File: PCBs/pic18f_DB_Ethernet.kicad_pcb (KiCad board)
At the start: 2 copper layers, 100 x 98 mm, 40 parts, among them J1 OC1, J2 PicKIT 3, J3 IC1, J4 FC1, J5 MC1, J6 DB9_Female, J7 DB9_Male, J8 RJ45, SW1 SW_DPDT_x2, SW2 PWR_SW, U1 pic18f45k20

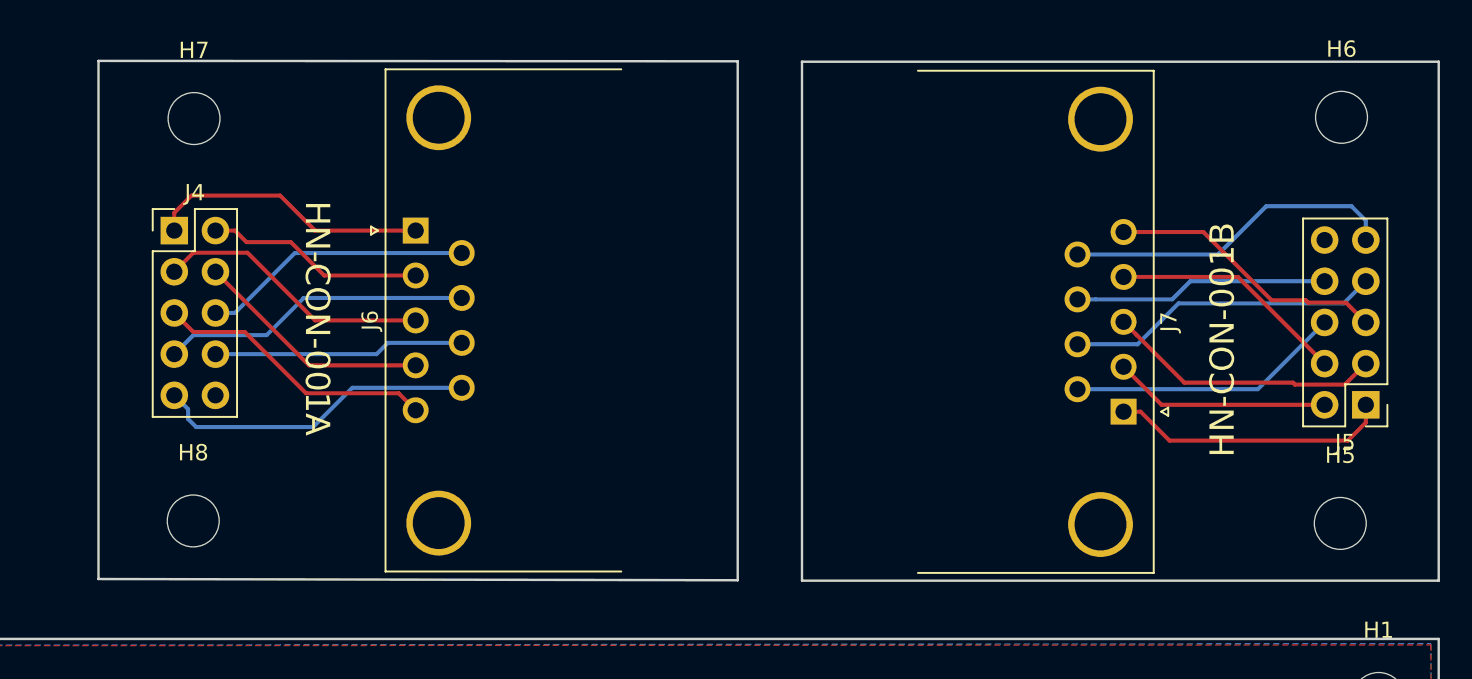
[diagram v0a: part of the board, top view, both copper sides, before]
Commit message: Restructed project
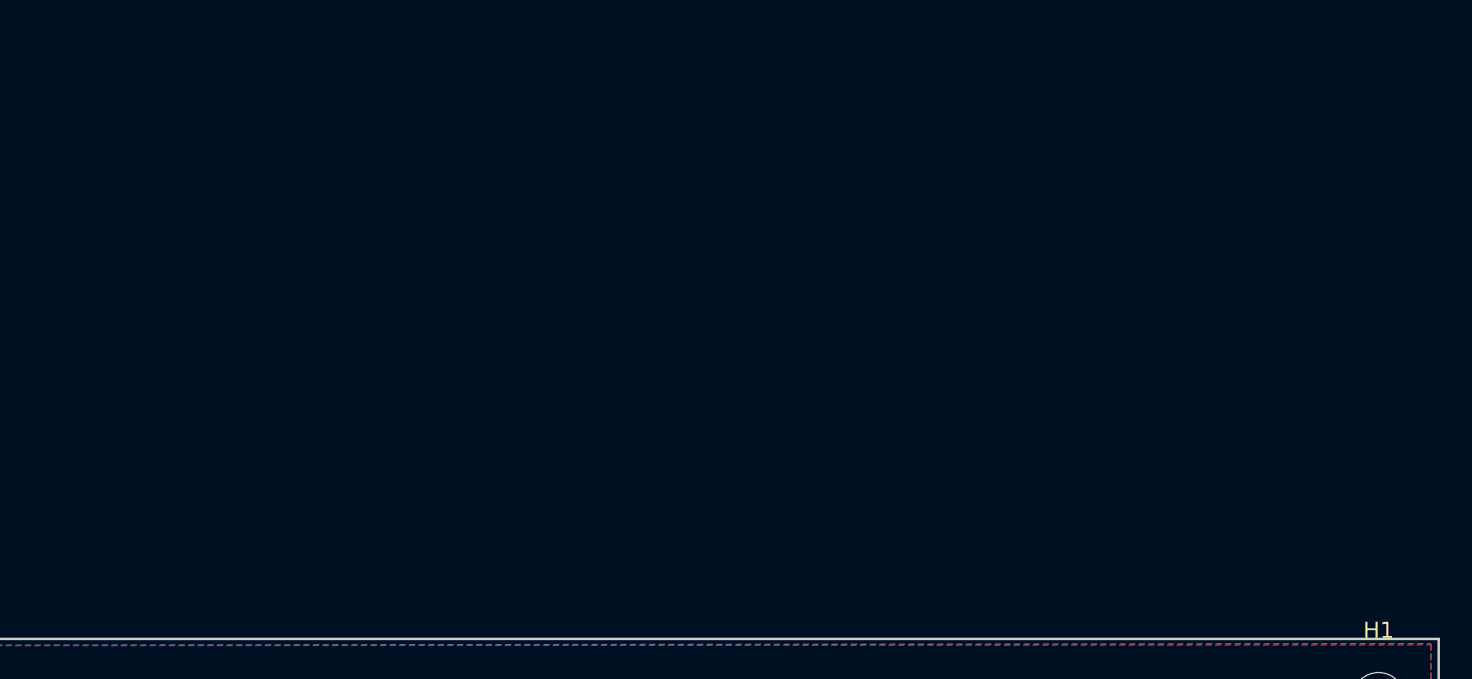
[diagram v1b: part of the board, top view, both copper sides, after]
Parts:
- removed H5, H6, H7, H8: MountingHole, MountingHole:MountingHole_3.2mm_M3
- removed J4: FC1, Connector_PinHeader_2.54mm:PinHeader_2x05_P2.54mm_Vertical
- removed J5: MC1, Connector_PinHeader_2.54mm:PinHeader_2x05_P2.54mm_Vertical
- removed J6: DB9_Female, Connector_Dsub:DSUB-9_Female_Horizontal_P2.77x2.84mm_EdgePinOffset9.90mm_Housed_MountingHolesOffset11.32mm
- removed J7: DB9_Male, Connector_Dsub:DSUB-9_Female_Horizontal_P2.77x2.84mm_EdgePinOffset9.90mm_Housed_MountingHolesOffset11.32mm
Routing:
- net M9: track 20.6 -> 0.00 mm
- net F9: track 19.9 -> 0.00 mm
- net M7: track 19.4 -> 0.00 mm
- net F7: track 19.2 -> 0.00 mm
- net F5: track 17.4 -> 0.00 mm
- net F1: track 17.3 -> 0.00 mm
- net M5: track 17.2 -> 0.00 mm
- net M1: track 17.2 -> 0.00 mm
- net F3: track 17.1 -> 0.00 mm
- net M3: track 17.1 -> 0.00 mm
- net M6: track 16.9 -> 0.00 mm
- net F6: track 16.7 -> 0.00 mm
- net M8: track 15.7 -> 0.00 mm
- net F8: track 15.5 -> 0.00 mm
- net F4: track 14.7 -> 0.00 mm
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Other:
- board size 100 x 98 mm -> 100 x 62.3 mm
- board text removed: "HN-CON-001A"
- board text removed: "HN-CON-001B"
